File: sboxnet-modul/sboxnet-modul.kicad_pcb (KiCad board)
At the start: 2 copper layers, 49.5 x 48.3 mm, 33 parts, among them J2 Conn_02x03_Odd_Even, J4 8P8C, J5 8P8C, J6 sboxnet-buchse_2x17, SW1 SW_Push, U1 MCP1703A-3302_SOT223, U2 MCP1703A-5002_SOT223, U3 SN65HVD230, U4 ATxmega128A4U-AU, Y1 16MHz

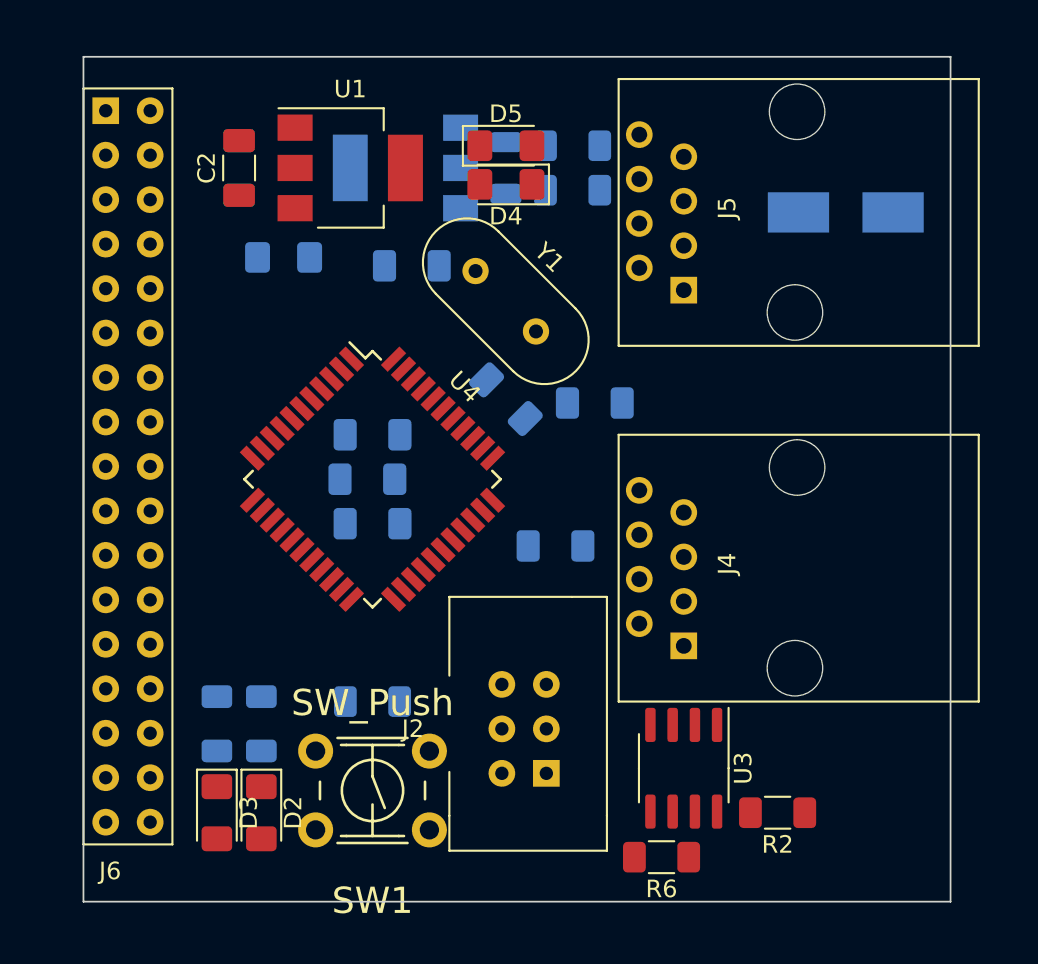
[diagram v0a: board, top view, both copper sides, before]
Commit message: sboxnet modul V6
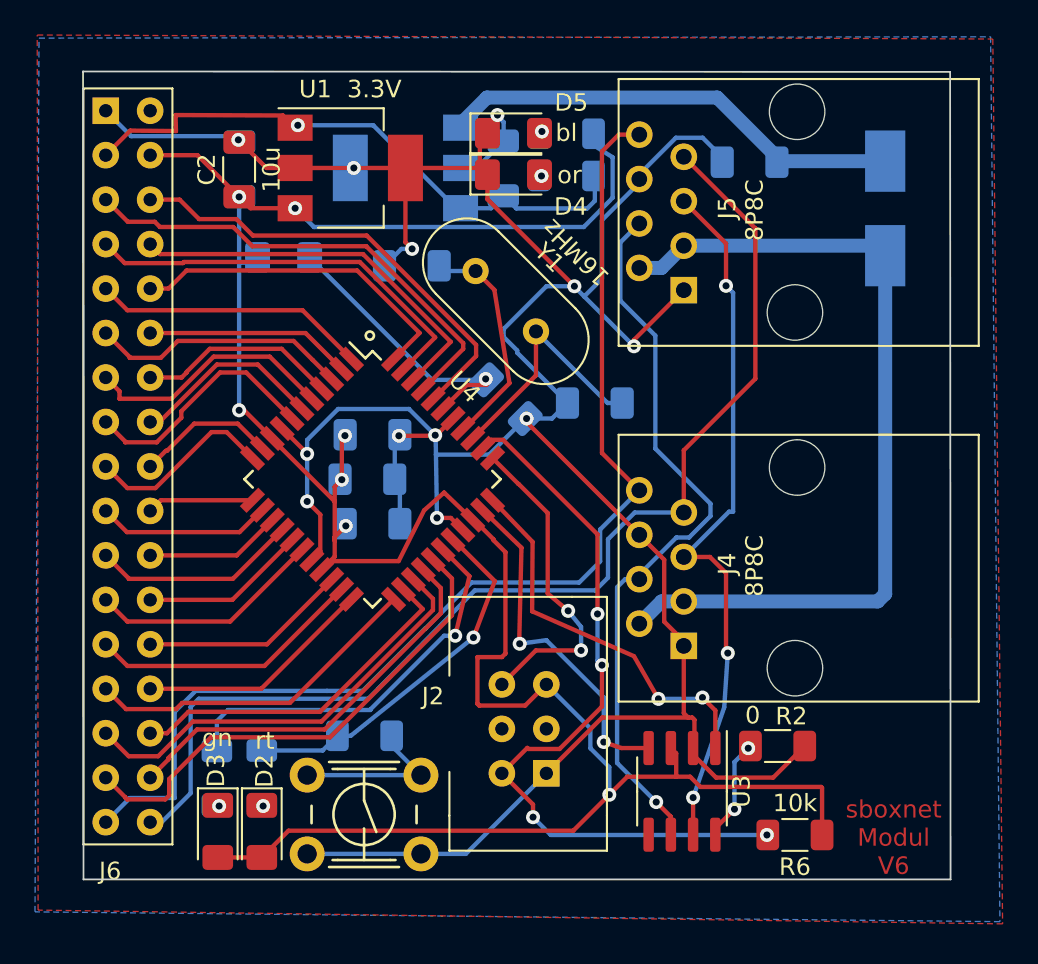
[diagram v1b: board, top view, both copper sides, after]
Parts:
- C3: footprint Capacitor_SMD:C_1206_3216Metric -> Capacitor_SMD:C_1206_3216Metric_Pad1.33x1.80mm_HandSolder
- L1: value Ferrit 60Ohm -> Ferrit
- U1  3.3V: renamed from U1
- U2  5V: renamed from U2
- moved C1 29.2 mm to (114.2, 80.9), turned to 0 degrees
- moved C5 28.1 mm to (85.1, 81.4), turned to -90 degrees
- moved R6 7.73 mm to (116.8, 119.4)
- moved R2 3.81 mm to (115.9, 114.3)
- moved R1 3.25 mm to (103.8, 79.3)
- moved R4 3.10 mm to (83.8, 116.1)
- moved R3 3.07 mm to (86.4, 116.1)
- moved D1 2.26 mm to (122.0, 83.6), turned to -90 degrees
- moved R5 2.01 mm to (92.3, 113.7)
- moved R7 1.76 mm to (103.8, 81.7)
- moved SW1 1.45 mm to (92.2, 118.2)
- moved U3 1.32 mm to (110.4, 116.9)
- moved D3 1.07 mm to (83.9, 119.2)
- moved D2 1.07 mm to (86.4, 119.2)
- moved D5 0.83 mm to (100.8, 79.3)
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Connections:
- D1 pad 2: Net-(D1-Pad2) -> +7V
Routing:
- net GND: track 0.00 -> 180.1 mm, vias 0 -> 12
- net +3.3V: track 0.00 -> 140.5 mm, vias 0 -> 7
- net DCC_A: track 0.00 -> 65.7 mm
- net DCC_B: track 0.00 -> 65.1 mm
- net +7V: track 0.00 -> 48.9 mm
- net PDICLK: track 0.00 -> 43.3 mm, vias 0 -> 4
- net CANL: track 0.00 -> 41.9 mm, vias 0 -> 1
- net CANH: track 0.00 -> 40.9 mm, vias 0 -> 3
- net +5V: track 0.00 -> 33.3 mm, vias 0 -> 1
- net PD7: track 0.00 -> 28.8 mm
- net PA1: track 0.00 -> 27.4 mm
- net Net-(C1-Pad2): track 0.00 -> 26.6 mm
- net PA0: track 0.00 -> 26.2 mm
- net PD5: track 0.00 -> 24.9 mm
- net PA3: track 0.00 -> 23.6 mm
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- added copper zone on B.Cu, net GND
- added copper zone on F.Cu, net GND
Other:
- board size 49.5 x 48.3 mm -> 49.6 x 46.2 mm
- board text added: "16MHz"
- board text added: "470"
- board text added: "bl"
- board text added: "gn"
- board text added: "or"
- board text added: "rt"
- board text added: "sboxnet Modul V6"
